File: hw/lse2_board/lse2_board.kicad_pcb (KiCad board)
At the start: 2 copper layers, 93.7 x 51.8 mm, 44 parts, among them IC1 DIGIT_DRIVER, IC2 DIGIT_DRIVER, J1 Conn_02x10_Odd_Even, J10 Conn_01x02, J2 Conn_02x10_Odd_Even, J3 Conn_02x10_Odd_Even, J4 Conn_02x10_Odd_Even, J5 Conn_02x05_Odd_Even, J7 Conn_01x05, J8 Conn_01x08, J9 Conn_02x05_Odd_Even, U1 NRF24L01_Breakout, U2 SN74LVC1G66DRLR

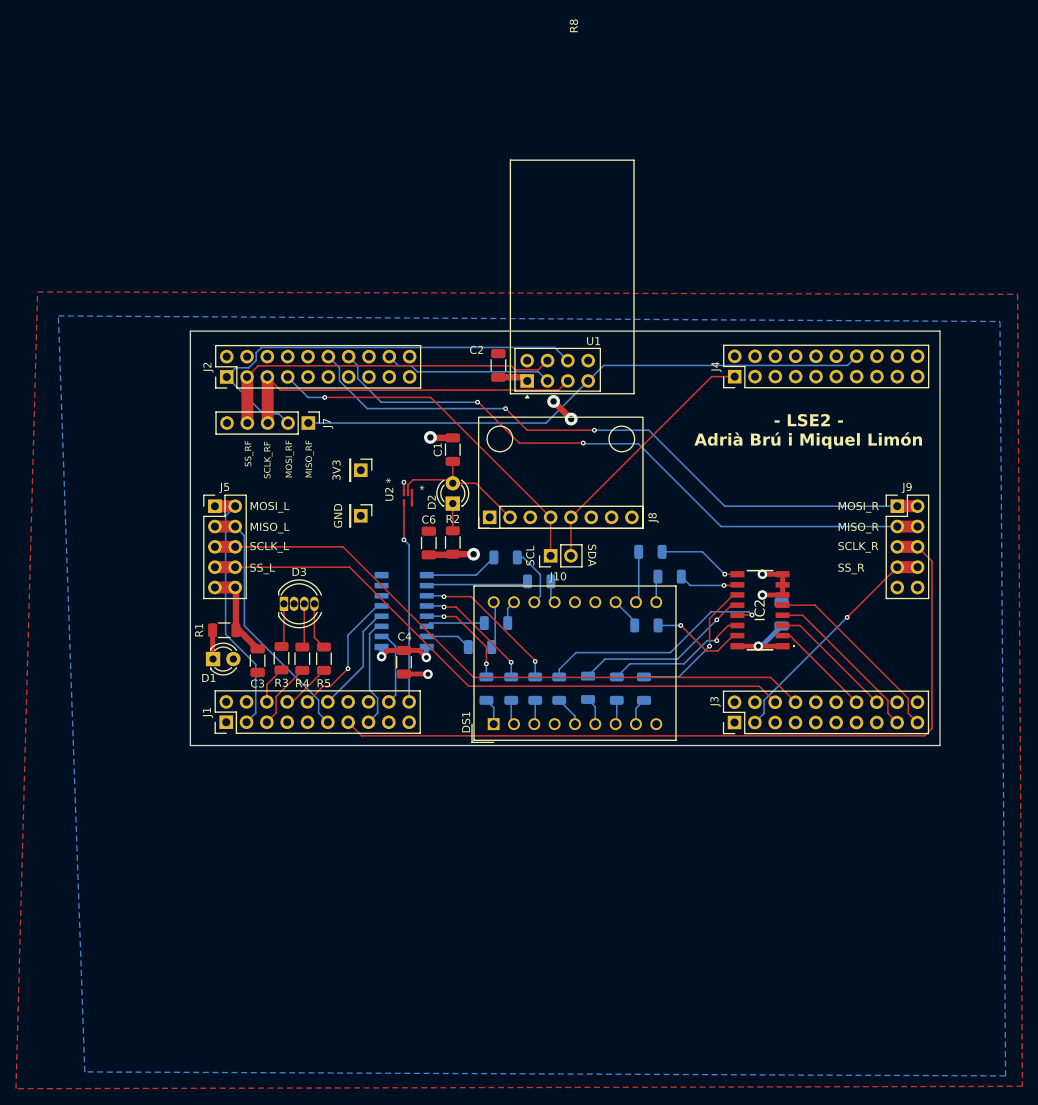
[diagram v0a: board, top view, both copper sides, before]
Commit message: nova placa (cal revisar)
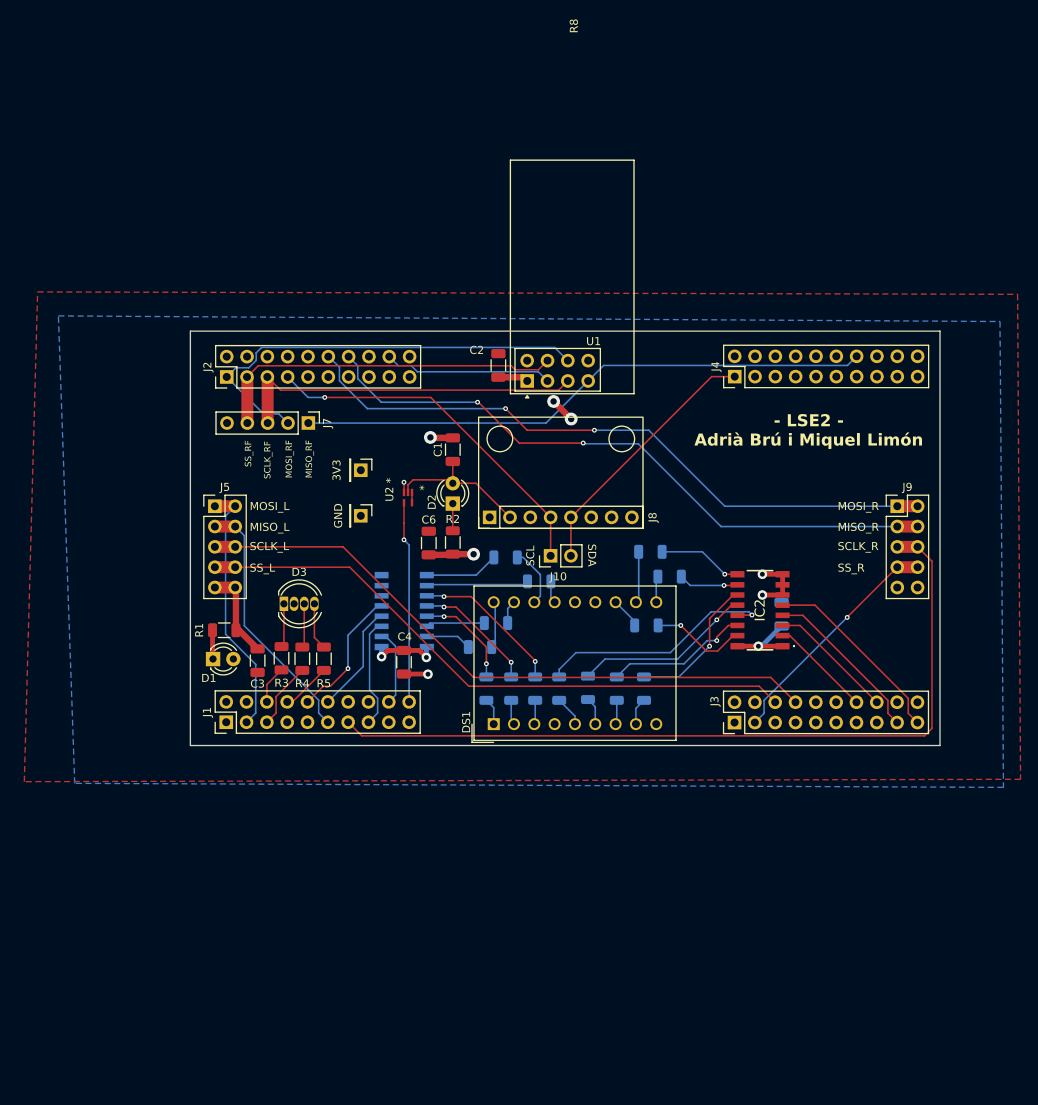
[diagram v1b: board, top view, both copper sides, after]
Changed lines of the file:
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@@
+	)
+	(segment
+		(start 108.235 59)
+		(end 108.235 60.714275)
+		(width 0.2)
+		(layer "B.Cu")
+		(net 47)
 	)
 	(segment
@@
 	)
 	(segment
-		(start 106.84 57.7)
-		(end 108.235 59.095)
-		(width 0.2)
-		(layer "B.Cu")
-		(net 47)
-	)
-	(segment
 		(start 140.1 66.9)
 		(end 146.9 66.9)
@@
 	)
 	(segment
-		(start 108.235 59.095)
-		(end 108.235 60.714275)
-		(width 0.2)
-		(layer "B.Cu")
-		(net 47)
-	)
-	(segment
 		(start 111.720725 64.2)
 		(end 129 64.2)
@@
 		(start 156.4 76.4)
 		(end 177.96 76.4)
+		(width 0.2)
+		(layer "B.Cu")
+		(net 47)
+	)
+	(segment
+		(start 106.84 57.7)
+		(end 108.235 59)
 		(width 0.2)
 		(layer "B.Cu")
@@
 		(polygon
 			(pts
-				(xy 70.500117 49.611733) (xy 193.000117 49.911733) (xy 193.600117 148.911733) (xy 67.800117 149.211733)
+				(xy 70.500117 49.611733) (xy 193.000117 49.911733) (xy 193.36751 110.531523) (xy 68.840626 110.828487)
 			)
 		)
@@
 		(polygon
 			(pts
-				(xy 73.100117 52.611733) (xy 190.800117 53.311733) (xy 191.500117 147.611733) (xy 76.400117 147.111733)
+				(xy 73.100117 52.611733) (xy 190.800117 53.311733) (xy 191.23238 111.543675) (xy 75.140447 111.039366)
 			)
 		)
